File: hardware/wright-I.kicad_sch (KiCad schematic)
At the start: 11 parts, among them U1 STM32F722RETx, U2 BQ25883RGER, U3 TPS63070RNMR, U4 LMR51430, U5 ICM-45686, U6 BMP580

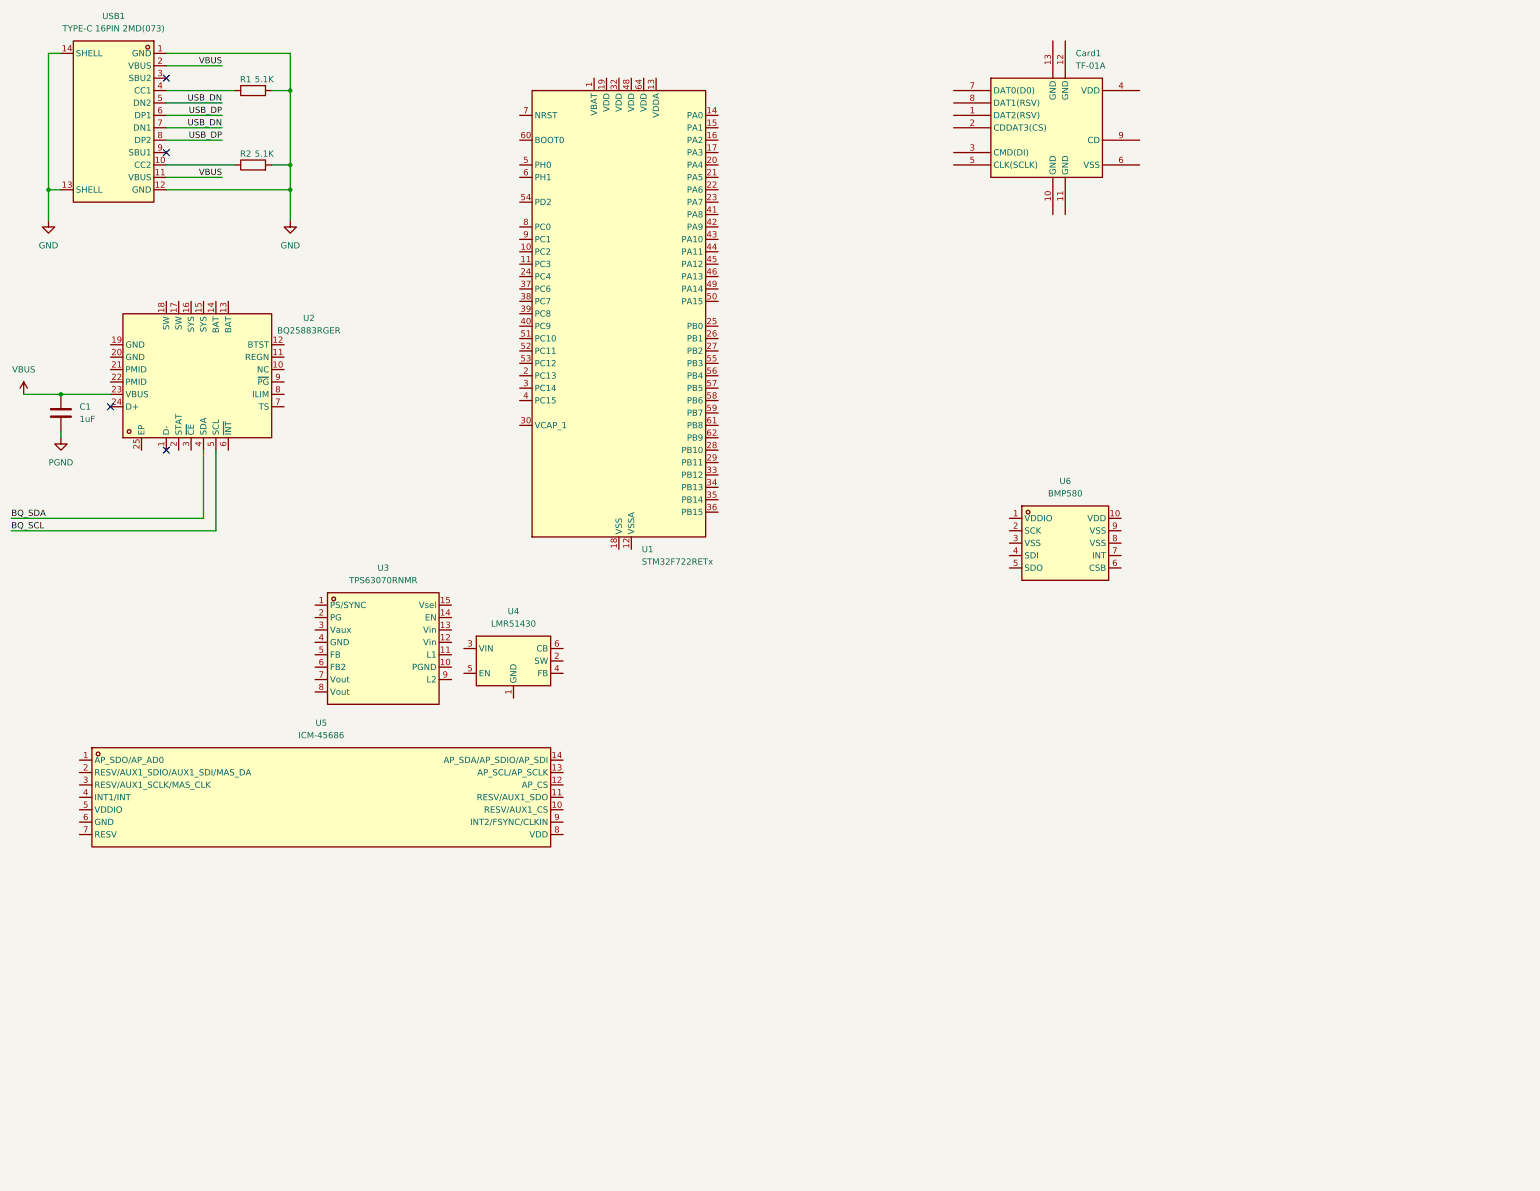
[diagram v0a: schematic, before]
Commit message: things
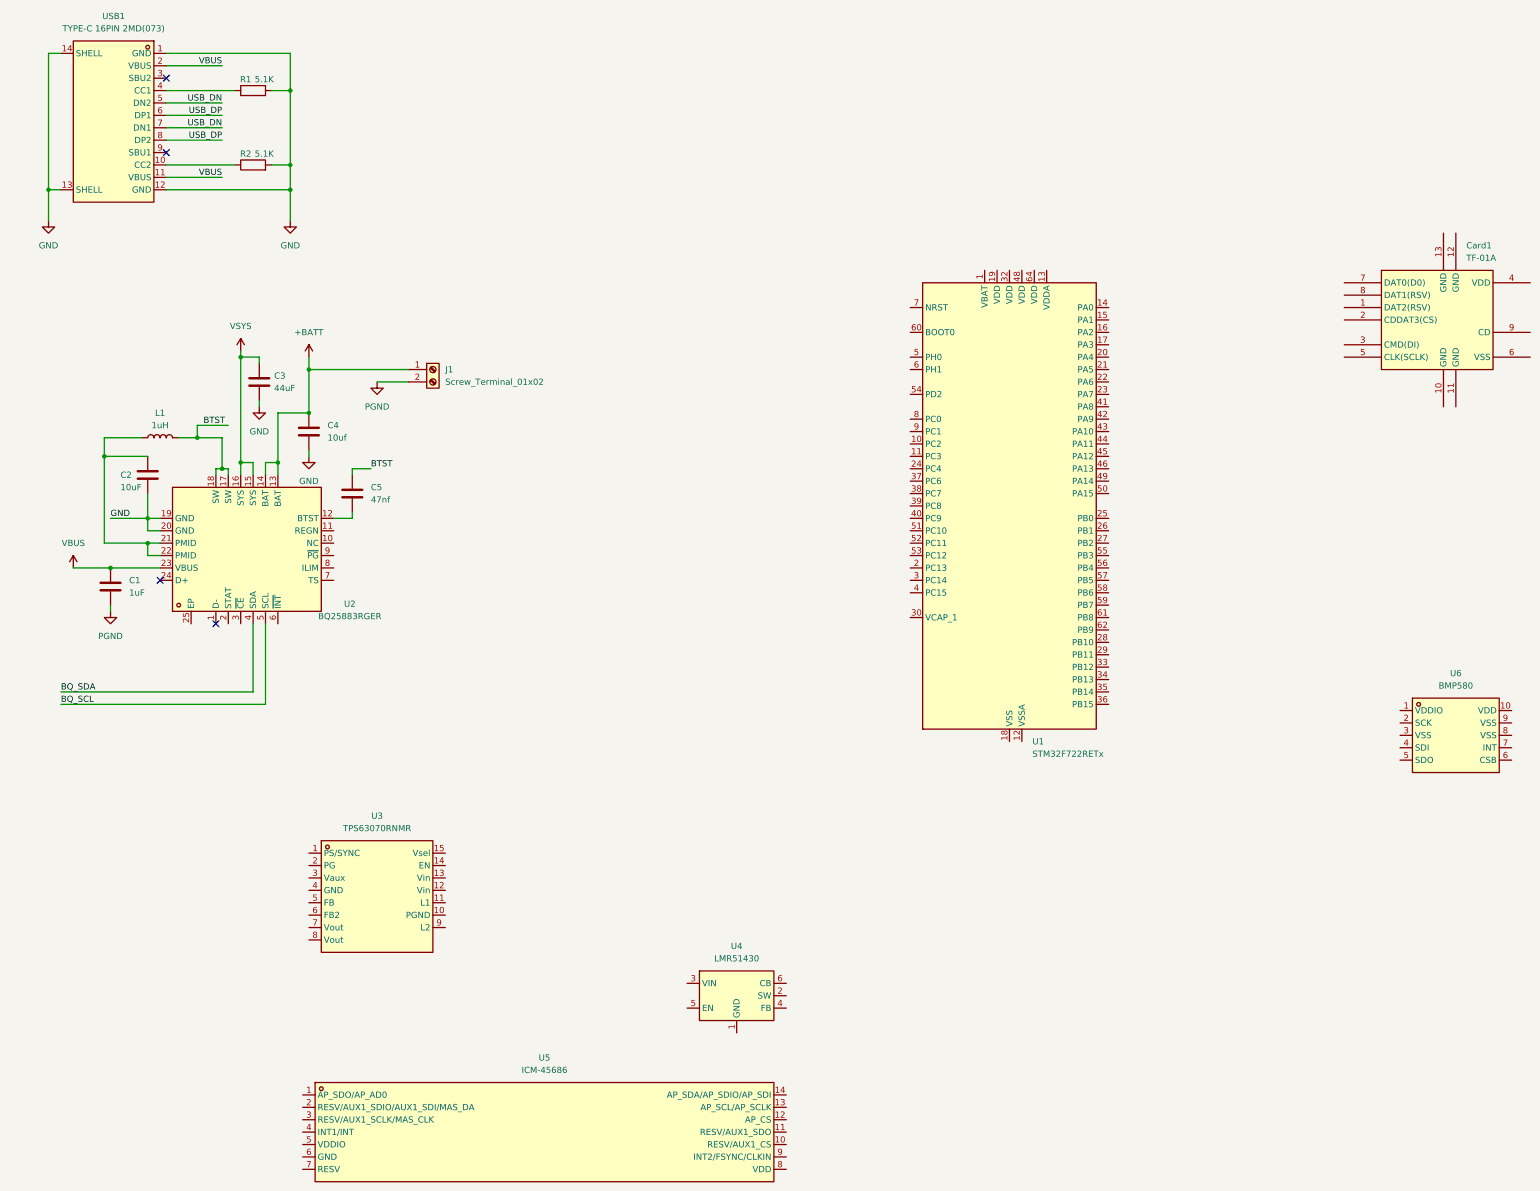
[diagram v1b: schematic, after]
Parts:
- added C2: 10uF, symbol Device:C
- added C3: 44uF, symbol Device:C
- added C4: 10uf, symbol Device:C
- added C5: 47nf, symbol Device:C
- added J1: Screw_Terminal_01x02, symbol Connector:Screw_Terminal_01x02
- added L1: 1uH, symbol Device:L
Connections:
- net GND: now also U2.19 (GND), U2.20 (GND), C2.2, C3.2, C4.2
- net PGND: now also J1.2 (Pin_2)
- net at U2.12 (BTST): now also C5.2
- net +BATT: now reaches U2.13 (BAT)
- net +BATT: now also U2.14 (BAT), C4.1, J1.1 (Pin_1)
- net VSYS: now reaches U2.15 (SYS)
- net VSYS: now also U2.16 (SYS), C3.1
- net BTST: now reaches U2.17 (SW)
- net BTST: now also U2.18 (SW), C5.1, L1.2
- net at U2.21 (PMID): now also U2.22 (PMID), C2.1, L1.1
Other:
- moved on the sheet: C1, Card1, U1, U2, U3, U4, U5, U6
